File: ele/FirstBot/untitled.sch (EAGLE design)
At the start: 58 parts, among them T1 BC337, T2 BC337, U1 ESP-WROOM-32, X0 POWER_IN, X1 USB-MICRO-B-BOTTOM

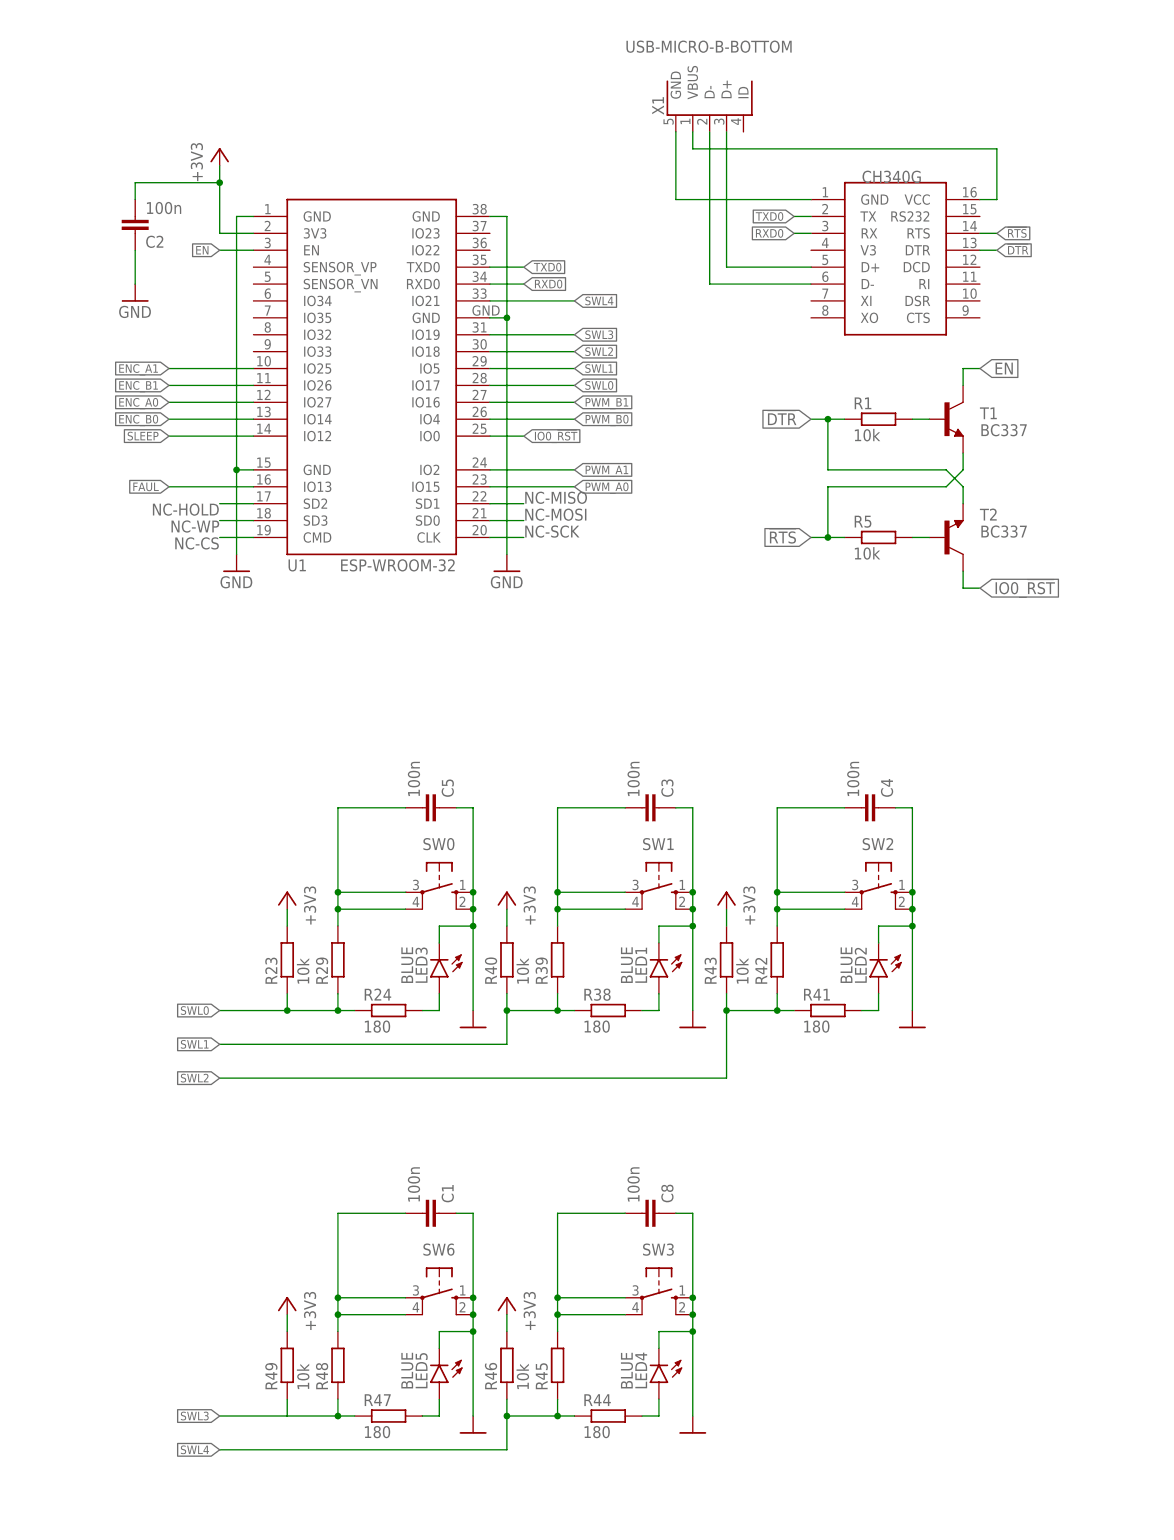
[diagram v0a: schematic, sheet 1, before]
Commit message: ESP32_wroom
CH340C
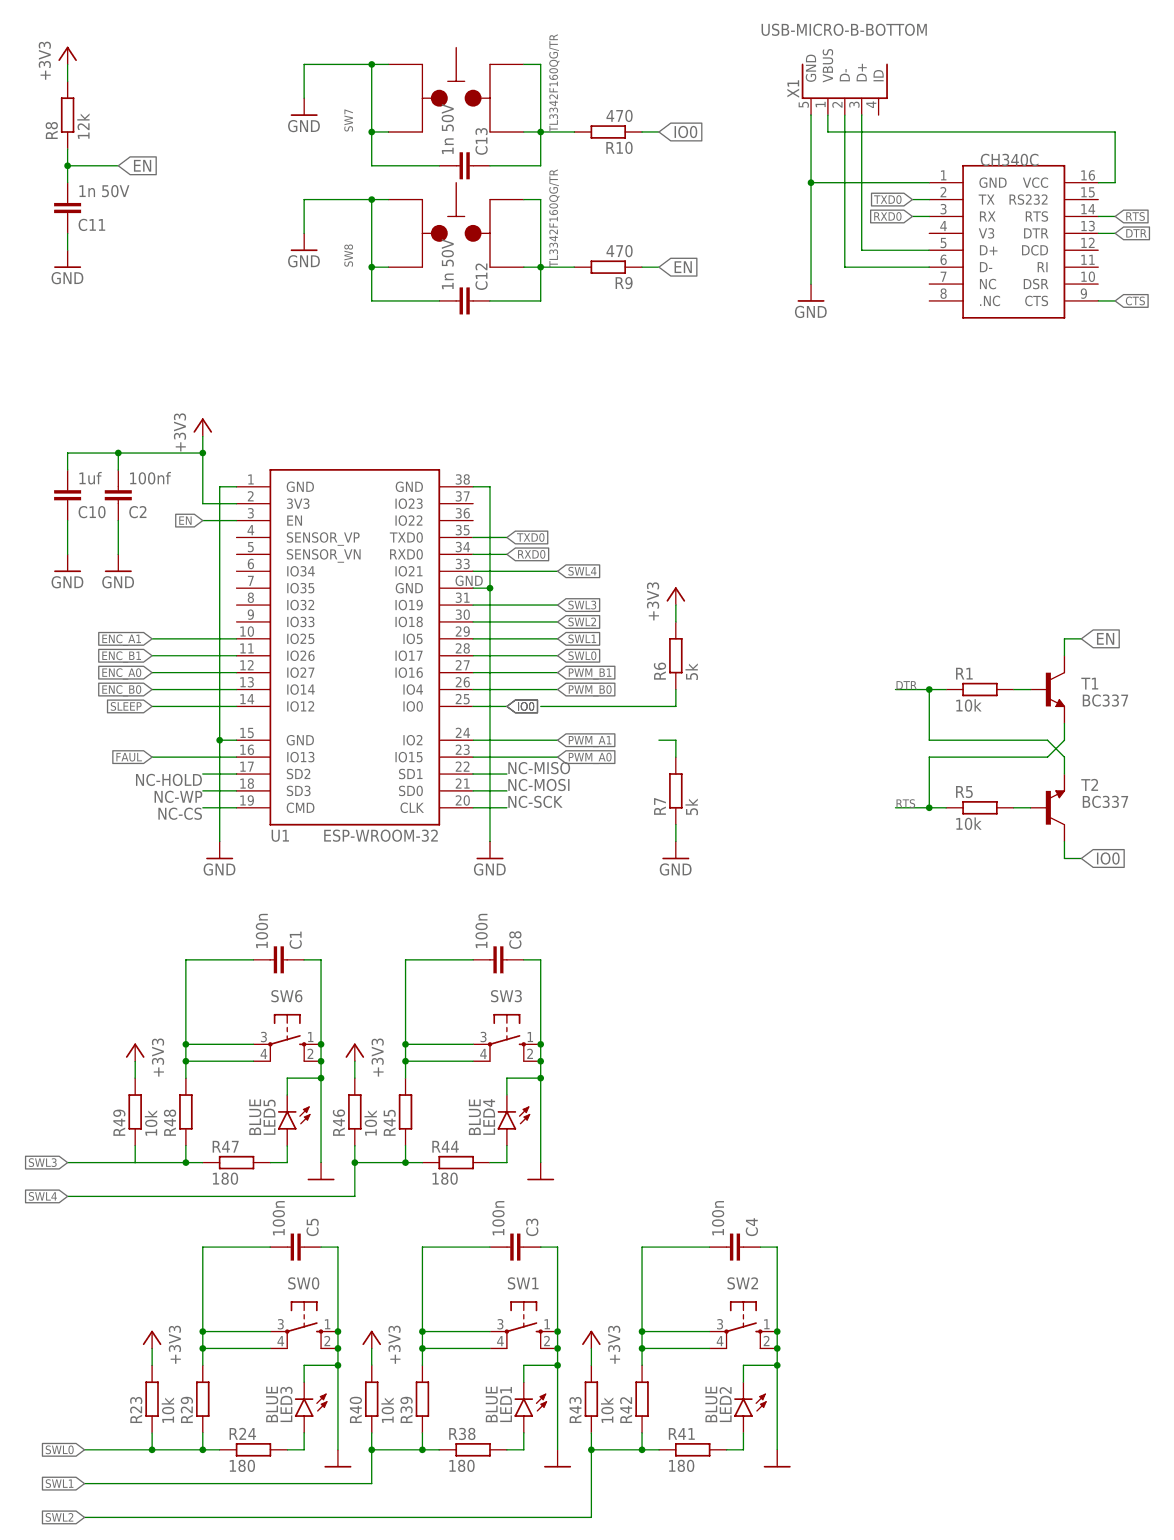
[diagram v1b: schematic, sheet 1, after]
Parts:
- added C10: 1uf, rcl_upravena:C-EUC0402
- added C11, C12, C13: 1n 50V, rcl_upravena:C-EUC0402
- added R10, R9: 470, rcl_upravena:R-EU_R0603
- added R6, R7: 5k, rcl_upravena:R-EU_R0603
- added R8: 12k, rcl_upravena:R-EU_R0603
- added SW7, SW8: TL3342F160QG/TR, Switch:TL3342F160QG/TR
- C2: value 100n -> 100nf
- CH1: value CH340G -> CH340C; device ch340g:CH340G -> ch340g:CH340C
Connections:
- net !DTR renamed DTR
- net !RTS renamed RTS
- removed net IO0_!RST: T2.C, U1.IO0
- new net CTS: CH1.CTS
- new net IO0: R10.1, R6.1, T2.C, U1.IO0
- new net N$7: C13.1, R10.2, SW7.1, SW7.2
- net +3V3: now also C10.2, R6.2, R8.2
- net EN: now also C11.2, R8.1, R9.1
- net GND: now also C10.1, C11.1, C12.2, C13.2, CH1.GND, R7.1, SW7.3, SW7.4, SW8.3, SW8.4, X1.GND
- net N$1: now also C12.1, R9.2, SW8.1, SW8.2; no longer CH1.GND, X1.GND
- net PWM_A1: now also R7.2
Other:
- moved on the sheet: C1, C2, C3, C4, C5, C8, LED1, LED2, LED3, LED4, LED5, R1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
